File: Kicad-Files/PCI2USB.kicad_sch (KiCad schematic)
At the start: 15 parts, among them U1 TPS61023

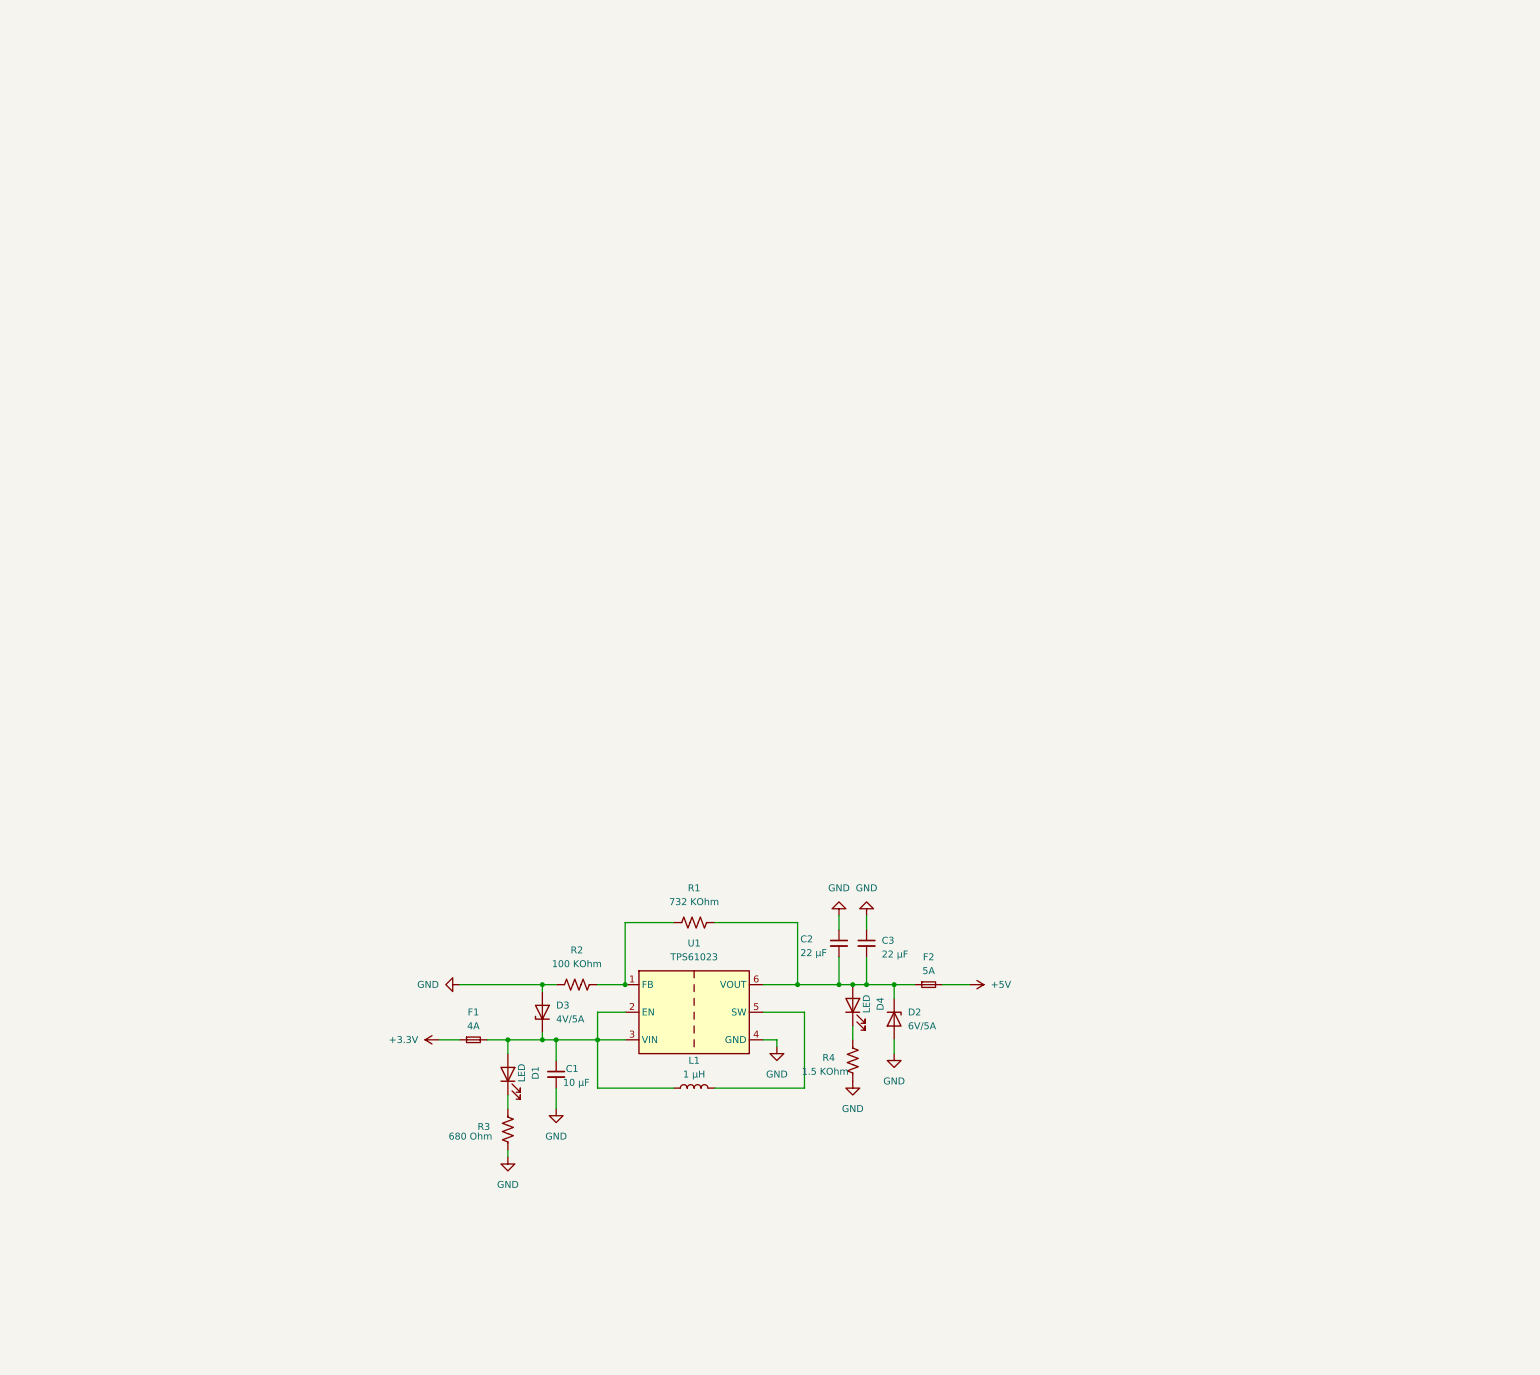
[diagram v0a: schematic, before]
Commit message: Updated schematics and board layout
Signed-off-by: Jakub Sobota <jakub.sobota@3mdeb.com>
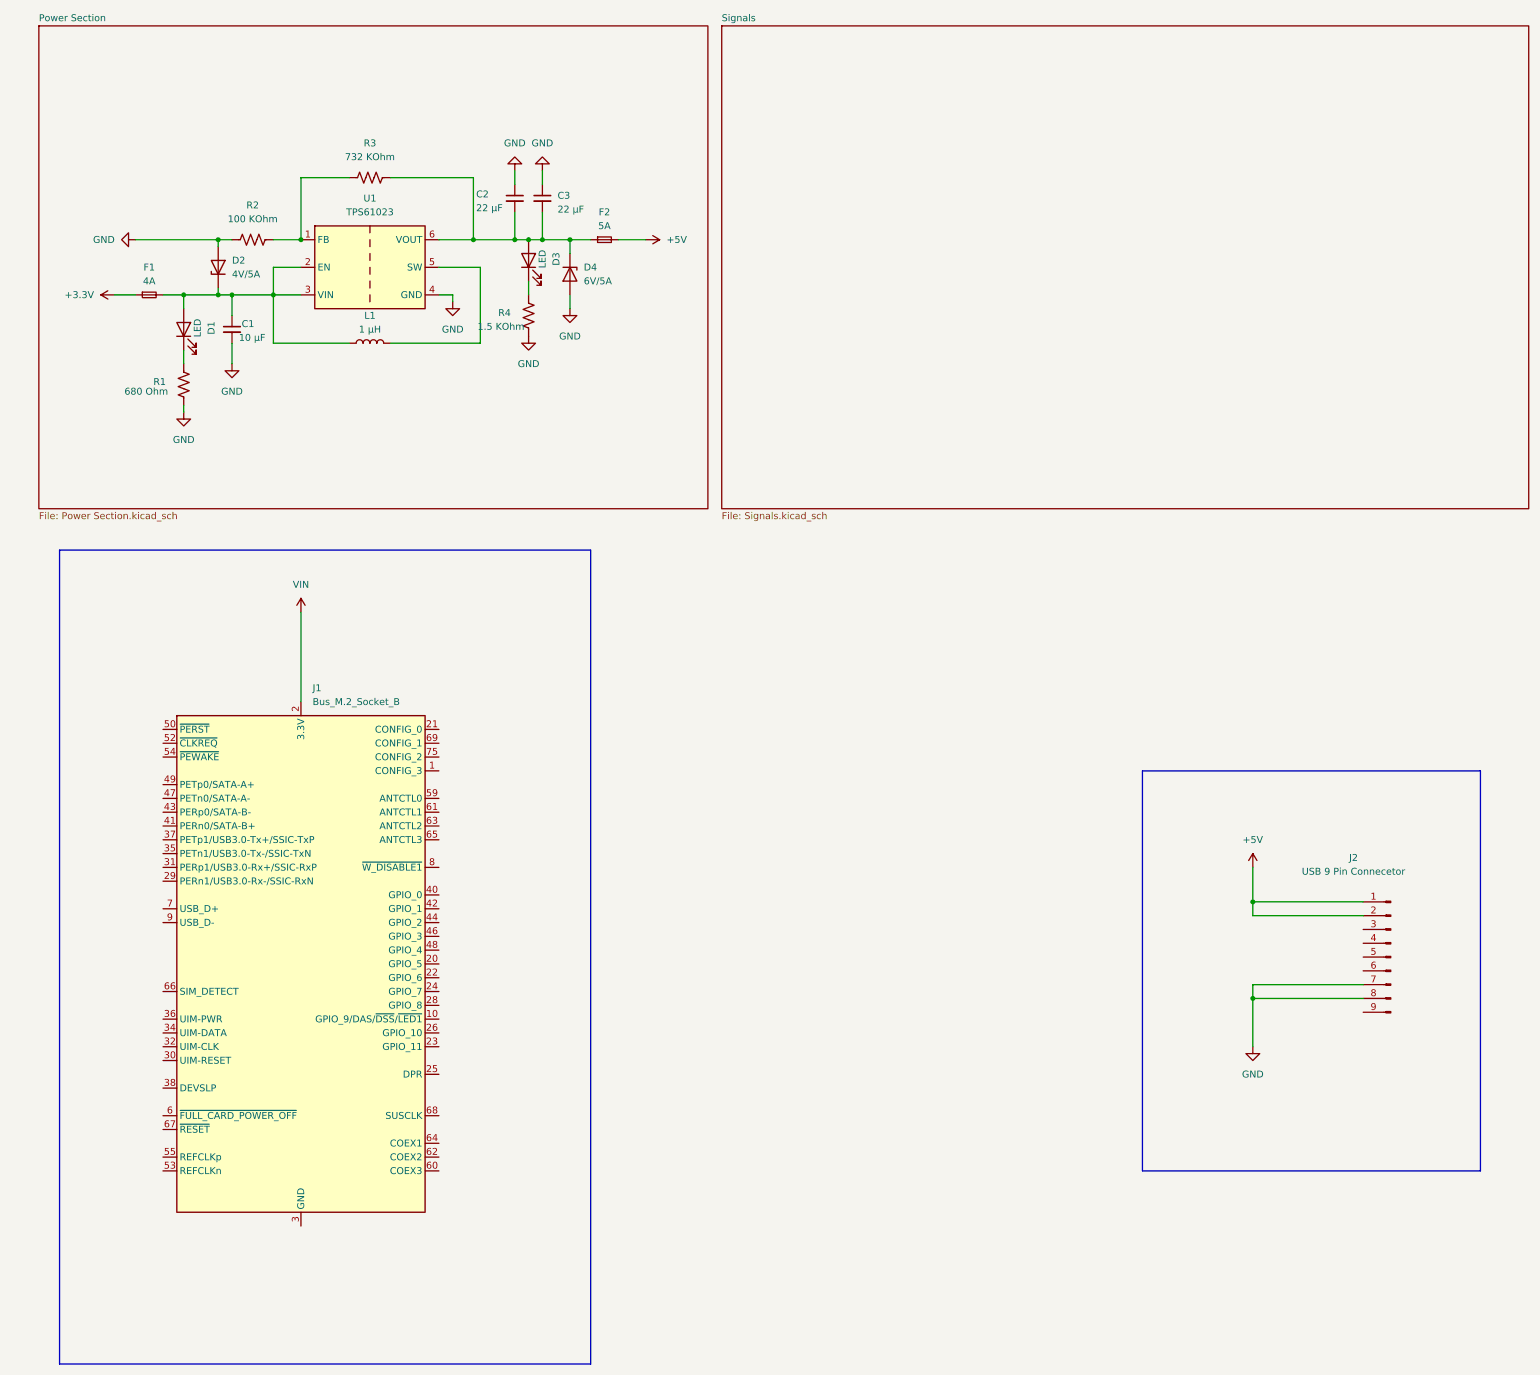
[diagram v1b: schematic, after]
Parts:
- removed D3: 4V/5A, Diode_SMD:D_SOD-523, symbol Diode:PTVS5V0Z1USK
- removed D4: LED, LED_SMD:LED_0603_1608Metric_Pad1.05x0.95mm_HandSolder, symbol Device:LED
- added D3: LED, LED_SMD:LED_0603_1608Metric_Pad1.05x0.95mm_HandSolder, symbol Device:LED
- added D4: 6V/5A, Diode_SMD:D_SOD-523, symbol Diode:PTVS5V0Z1USK
- added J1: Bus_M.2_Socket_B, symbol Connector:Bus_M.2_Socket_B
- added J2: USB 9 Pin Connecetor, Connectors:USB 9 Pin internal header, symbol Connector:Conn_01x09_Pin
- D2: value 6V/5A -> 4V/5A
- R1: value 732 KOhm -> 680 Ohm; footprint Resistor_SMD:R_0603_1608Metric_Pad0.98x0.95mm_HandSolder -> Resistor_SMD:R_0201_0603Metric_Pad0.64x0.40mm_HandSolder
- R3: value 680 Ohm -> 732 KOhm; footprint Resistor_SMD:R_0201_0603Metric_Pad0.64x0.40mm_HandSolder -> Resistor_SMD:R_0603_1608Metric_Pad0.98x0.95mm_HandSolder
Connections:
- net +5V: now also J2.1 (Pin_1), J2.2 (Pin_2)
- net GND: now also R1.2, D4.2 (A), J2.7 (Pin_7), J2.8 (Pin_8); no longer R3.2
- net at C2.2, C3.2, F2.1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: now also R3.2, D3.2 (A), D4.1 (K); no longer D2.1 (K), R1.2
- net at C1.1, D1.2 (A), F1.2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: now also D2.1 (K)
- net at R4.1: now also D3.1 (K)
- net at R2.2, U1.1 (FB): now also R3.1; no longer R1.1
- net at D1.1 (K): now also R1.1; no longer R3.1
- new net: J1.11 (GND), J1.27 (GND), J1.3 (GND), J1.33 (GND), J1.39 (GND), J1.45 (GND), J1.5 (GND), J1.51 (GND), J1.57 (GND), J1.71 (GND), J1.73 (GND)
- new net VIN: J1.2 (3.3V), J1.4 (3.3V), J1.70 (3.3V), J1.72 (3.3V), J1.74 (3.3V)
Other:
- added sheet Power Section (Power Section.kicad_sch)
- added sheet Signals (Signals.kicad_sch)
- title: m2 PCIe to USB Converter -> PCI2USB

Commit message: Created schematics for 1.1V circuit
Signed-off-by: Jakub Sobota <jakub.sobota@3mdeb.com>
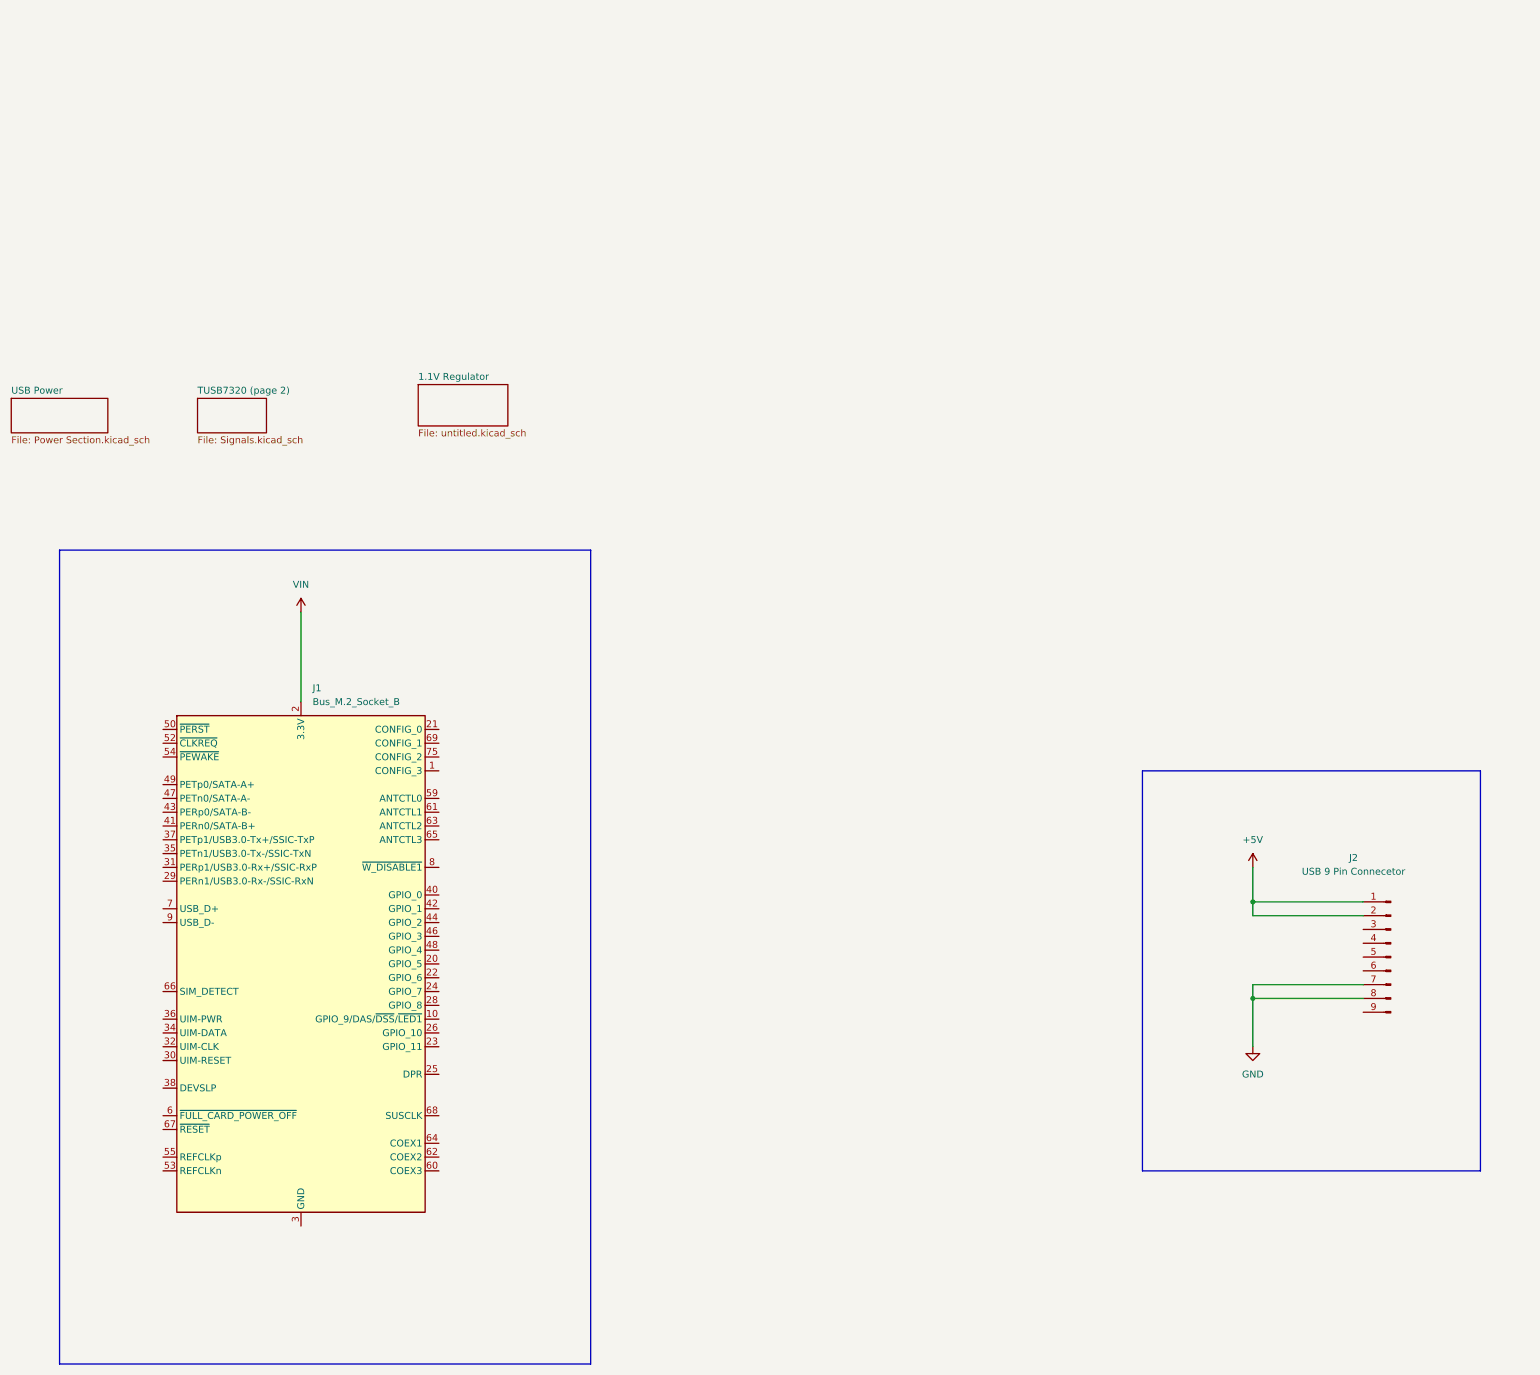
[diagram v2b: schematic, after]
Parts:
- removed C1: 10 μF, Capacitor_SMD:C_0805_2012Metric_Pad1.18x1.45mm_HandSolder, symbol Device:C_Small
- removed C2, C3: 22 μF, Capacitor_SMD:C_1206_3216Metric_Pad1.33x1.80mm_HandSolder, symbol Device:C_Small
- removed D1, D3: LED, LED_SMD:LED_0603_1608Metric_Pad1.05x0.95mm_HandSolder, symbol Device:LED
- removed D2: 4V/5A, Diode_SMD:D_SOD-523, symbol Diode:PTVS5V0Z1USK
- removed D4: 6V/5A, Diode_SMD:D_SOD-523, symbol Diode:PTVS5V0Z1USK
- removed F1: 4A, Fuse:Fuse_0603_1608Metric_Pad1.05x0.95mm_HandSolder, symbol Device:Fuse_Small
- removed F2: 5A, Fuse:Fuse_0603_1608Metric_Pad1.05x0.95mm_HandSolder, symbol Device:Fuse_Small
- removed L1: 1 μH, Inductor_SMD:L_Chilisin_BMRx00050515, symbol Device:L
- removed R1: 680 Ohm, Resistor_SMD:R_0201_0603Metric_Pad0.64x0.40mm_HandSolder, symbol Device:R_US
- removed R2: 100 KOhm, Resistor_SMD:R_0603_1608Metric_Pad0.98x0.95mm_HandSolder, symbol Device:R_US
- removed R3: 732 KOhm, Resistor_SMD:R_0603_1608Metric_Pad0.98x0.95mm_HandSolder, symbol Device:R_US
- removed R4: 1.5 KOhm, Resistor_SMD:R_0201_0603Metric_Pad0.64x0.40mm_HandSolder, symbol Device:R_US
- removed U1: TPS61023, DC-DC_Converter:TPS61023, symbol TPS61023:TPS61023
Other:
- sheet Power Section renamed USB Power
- sheet Signals renamed TUSB7320 (page 2)
- added sheet 1.1V Regulator (untitled.kicad_sch)
